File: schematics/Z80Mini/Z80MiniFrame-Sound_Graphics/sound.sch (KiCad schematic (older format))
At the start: 17 parts, among them U7 AY-3-8910, U8 74LS02, U9 LM386, X1 ACO-2MHz

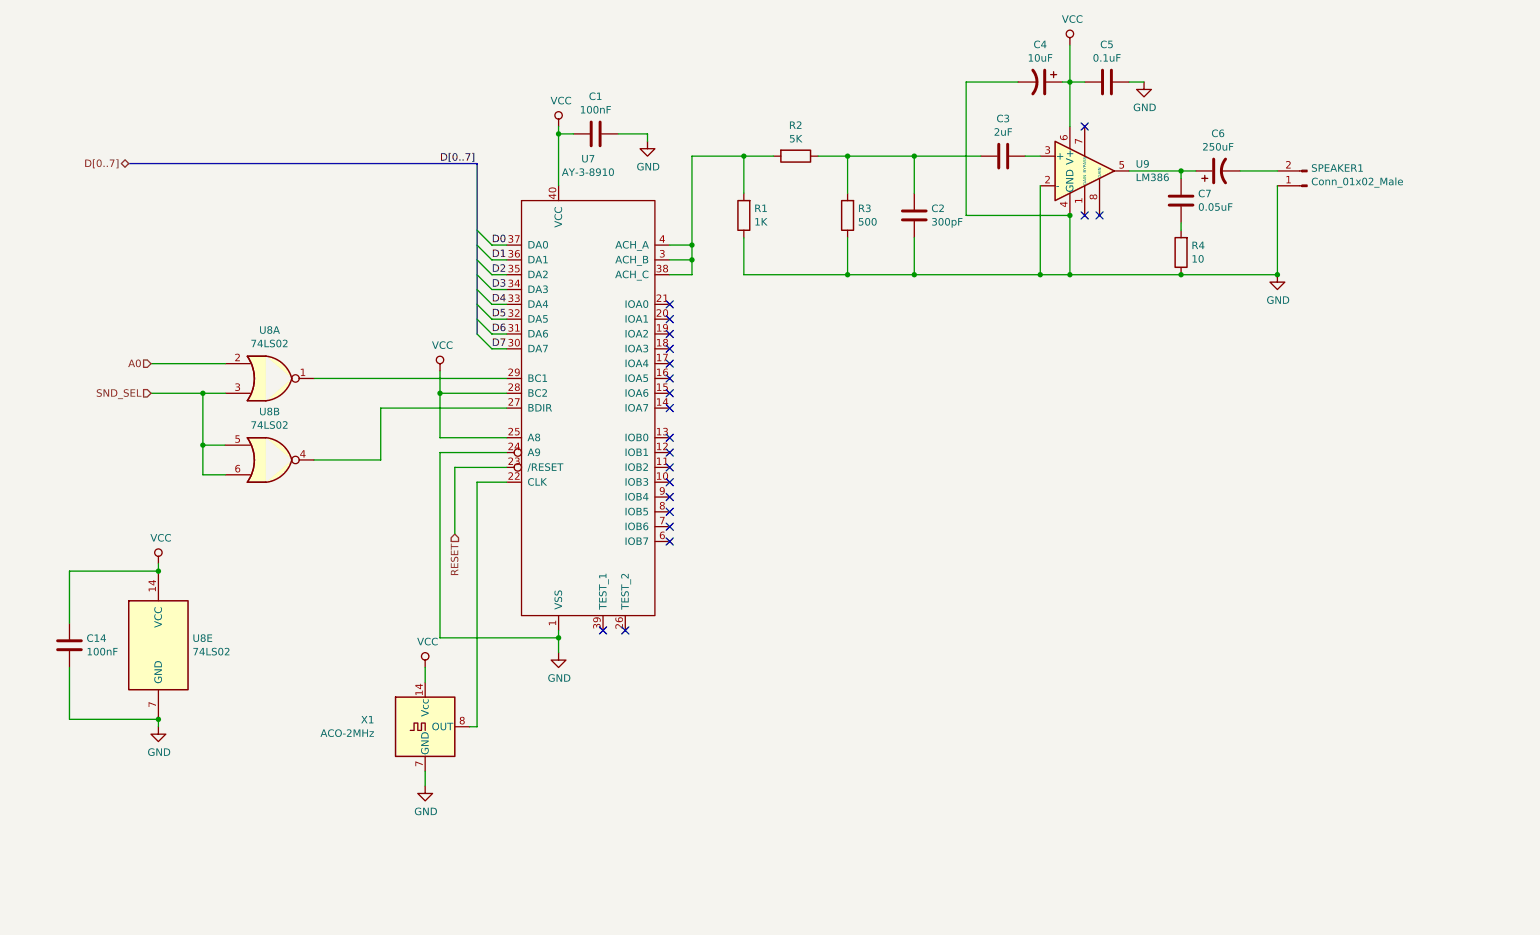
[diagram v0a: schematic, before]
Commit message: Latest modifications on Graphics-Sound card
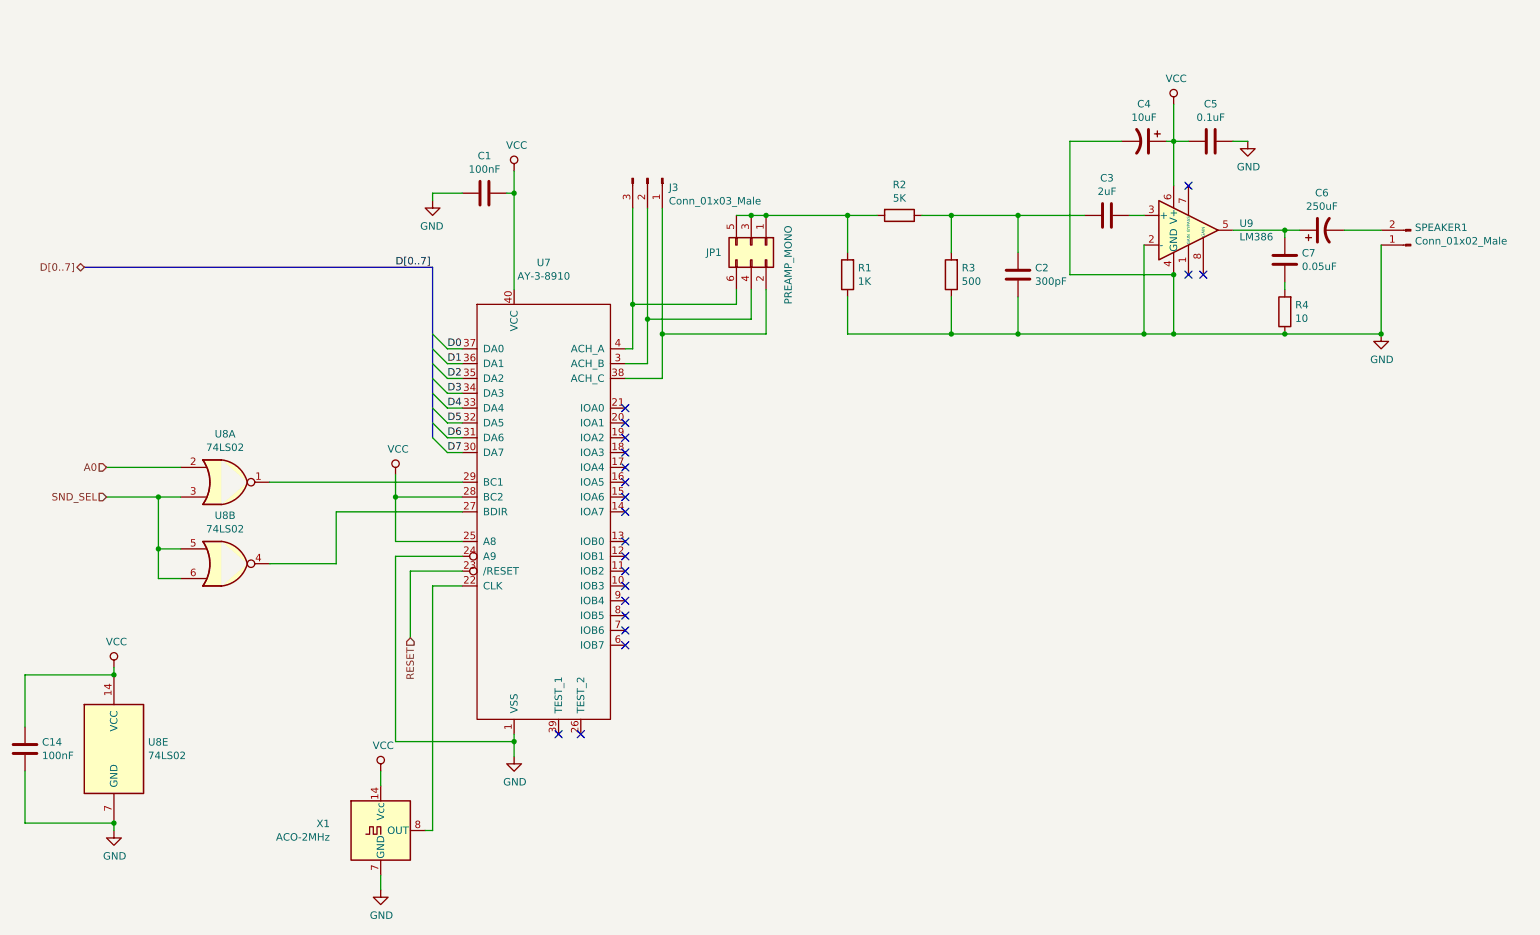
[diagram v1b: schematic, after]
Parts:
- added J3: Conn_01x03_Male, Connector_PinHeader_2.00mm:PinHeader_1x03_P2.00mm_Vertical, symbol Connector:Conn_01x03_Male
- added JP1: PREAMP_MONO, Connector_PinHeader_2.00mm:PinHeader_2x03_P2.00mm_Vertical, symbol Connector_Generic:Conn_02x03_Odd_Even
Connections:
- new net: J3.2 (Pin_2), JP1.4 (Pin_4), U7.3 (ACH_B)
- new net: J3.1 (Pin_1), JP1.2 (Pin_2), U7.38 (ACH_C)
- new net: J3.3 (Pin_3), JP1.6 (Pin_6), U7.4 (ACH_A)
- new net: JP1.1 (Pin_1), JP1.3 (Pin_3), JP1.5 (Pin_5), R1.2, R2.2
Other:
- moved on the sheet: C1, C14, C2, C3, C4, C5, C6, C7, R1, R2, R3, R4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
